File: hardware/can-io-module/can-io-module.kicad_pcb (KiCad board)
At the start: 2 copper layers, 96 x 86 mm, 95 parts, among them J1 ECU_FCI_24P_RightAngle, J2 SWD_1x05_P2.54mm_DNP, Q1 60V P-channel reverse polarity, Q4 60V logic N-MOS RELAY1, Q5 60V logic N-MOS RELAY2, U1 STM32G0B1CBT6, U10 MAX31855KASA+, U11 Schmitt Flex front end, U2 LMR16006Y-Q1, U3 3V3 LDO 300mA, U4 SENSOR_5V load switch, U5 74HCT4051 1K excitation, U6 74HCT4051 4K7 excitation, U7 L9613, U8 TJA1051T/3, U9 TLV9002-Q1

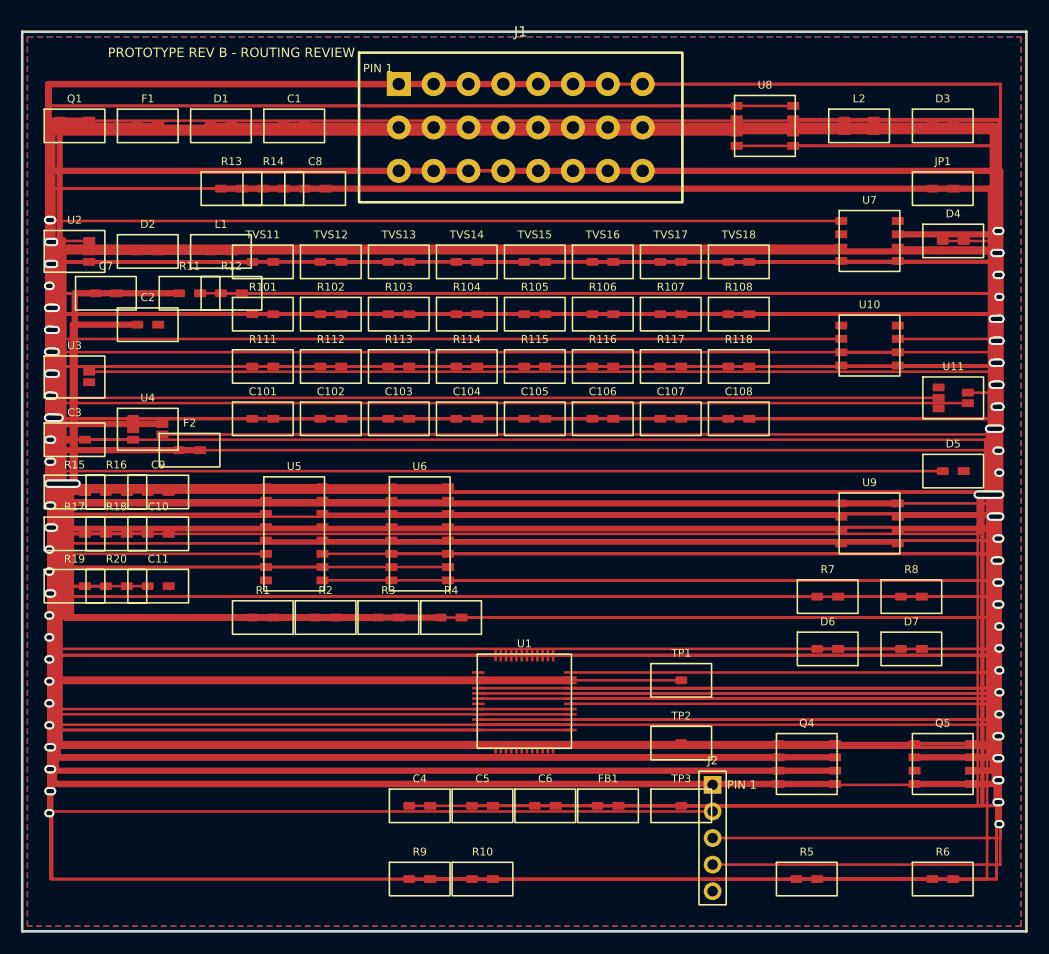
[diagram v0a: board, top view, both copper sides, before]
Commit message: chore: store verified CAN IO route [skip ci]
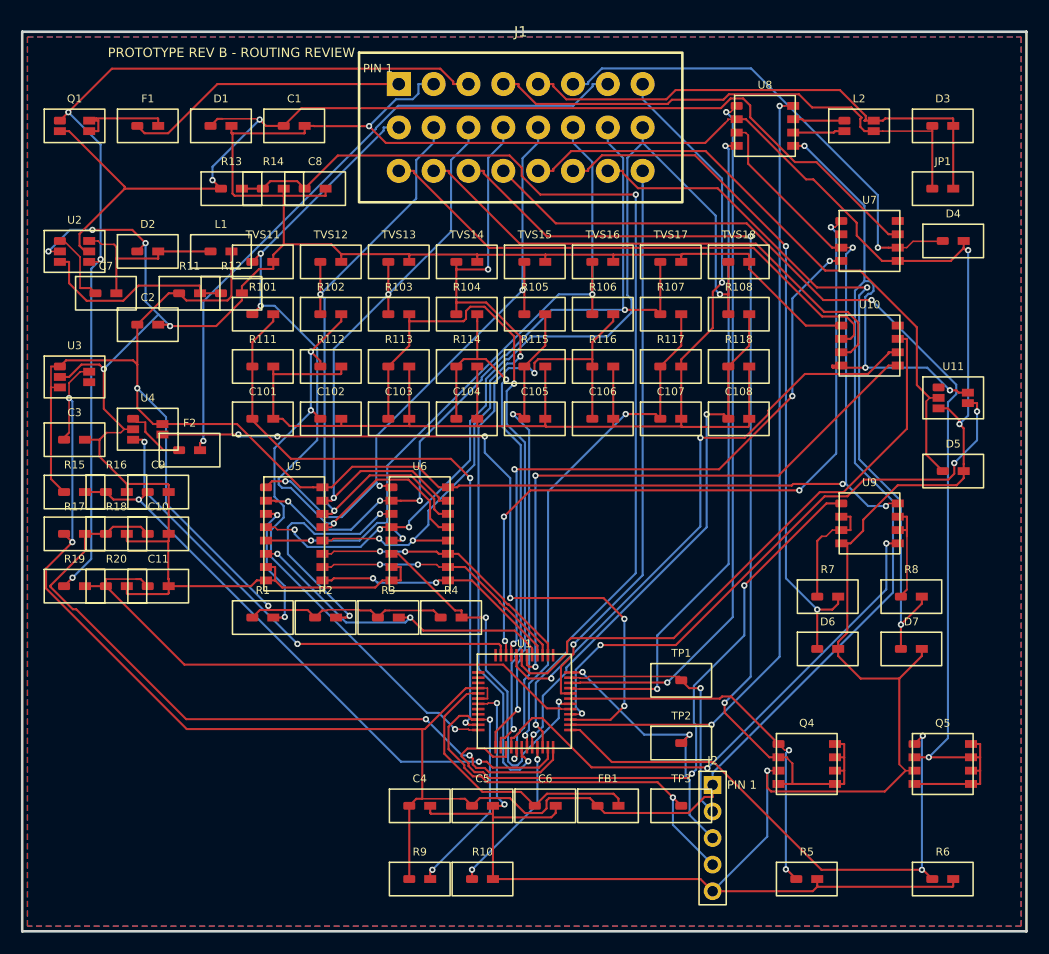
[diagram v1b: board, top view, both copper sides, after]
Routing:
- net +3V3: track 901.4 -> 225.2 mm, vias 13 -> 5
- net RELAY_OUT1: track 704.0 -> 99.5 mm, vias 7 -> 2
- net VBAT_PROTECTED: track 600.5 -> 108.4 mm, vias 6 -> 2
- net POWER_GND: track 0.00 -> 473.2 mm, vias 0 -> 11
- net +5V: track 649.1 -> 209.8 mm, vias 16 -> 5
- net V5_MON: track 413.6 -> 57.8 mm, vias 4 -> 2
- net AOUT1_OP: track 319.1 -> 11.1 mm, vias 3 -> 0
- net AIN2: track 363.2 -> 62.3 mm, vias 5 -> 2
- net CAN_L: track 350.0 -> 49.2 mm, vias 4 -> 0
- net BUCK_FB: track 314.2 -> 19.4 mm, vias 3 -> 0
- net AIN4: track 337.8 -> 66.3 mm, vias 5 -> 4
- net ADC_IN1: track 311.5 -> 58.9 mm, vias 4 -> 2
- net AIN6: track 318.0 -> 69.1 mm, vias 5 -> 3
- net ADC_IN8: track 289.7 -> 51.9 mm, vias 4 -> 2
- net AIN7: track 288.3 -> 74.2 mm, vias 5 -> 4
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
